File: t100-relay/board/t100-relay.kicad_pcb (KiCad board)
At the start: 2 copper layers, 34.5 x 99.5 mm, 14 parts, among them J1 T100-IN, J2 T100-OUT, J3 Conn_01x02_Female, J4 Conn_01x02_Female, K1 RELAY_2, Q1 BC817, U1 ATSAMD09C13A-SS, X1 SWD

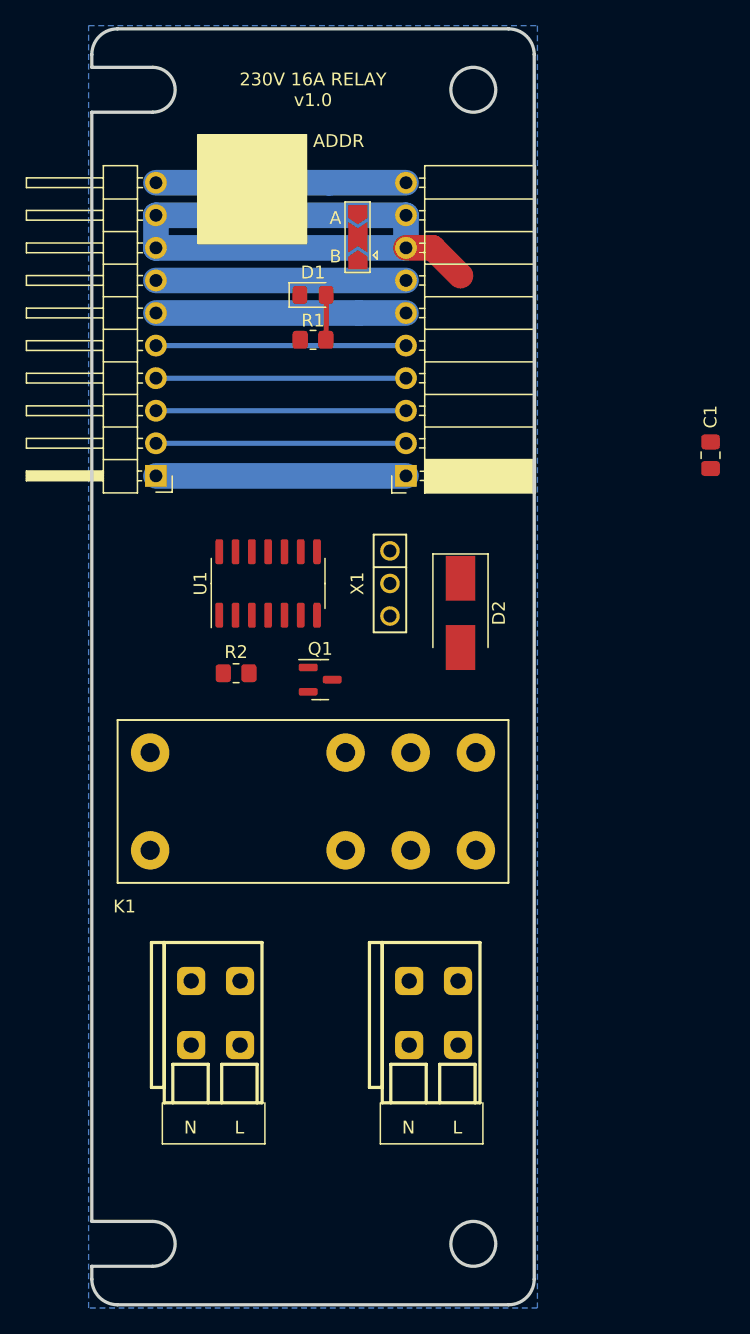
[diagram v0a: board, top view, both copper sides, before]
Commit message: WIP
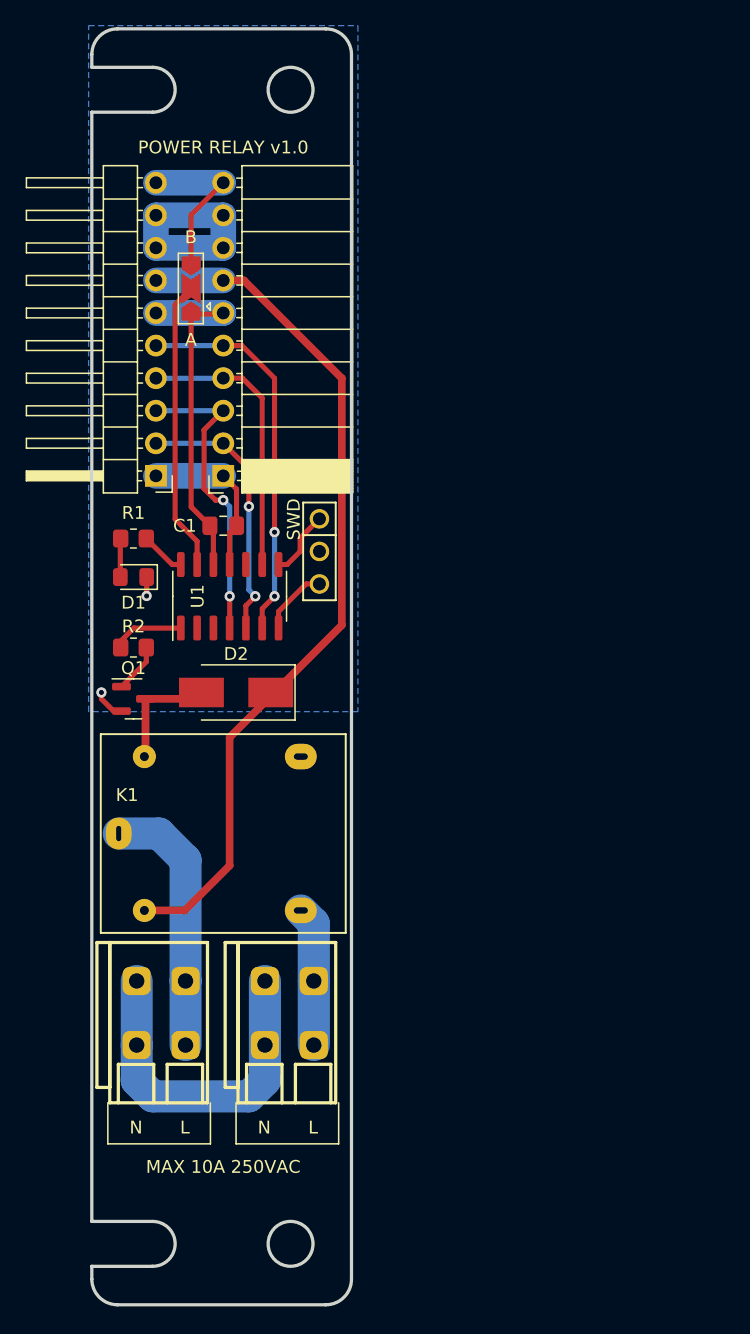
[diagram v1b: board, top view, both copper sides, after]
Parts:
- K1: value RELAY_2 -> RELAY_1; footprint Drake:RT314_Relay -> Drake:SRD_C_Relay
- moved C1 38.4 mm to (93.0, 89.0), turned to 0 degrees
- moved D1 26.1 mm to (86.0, 93.0), turned to 180 degrees
- moved R1 20.9 mm to (86.0, 90.0), turned to 0 degrees
- moved D2 18.6 mm to (94.0, 102.0), turned to 180 degrees
- moved Q1 14.6 mm to (86.0, 102.5)
- moved J2 14.2 mm to (93.0, 85.1)
- moved JP1 13.6 mm to (90.5, 70.5)
- moved J4 11.2 mm to (96.2, 124.5)
- moved R2 8.25 mm to (86.0, 98.5)
- moved X1 6.04 mm to (100.5, 91.0)
- moved J3 4.25 mm to (86.2, 124.5)
- moved U1 3.16 mm to (93.5, 94.5)
- moved K1 2.78 mm to (84.8, 113.0)
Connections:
- K1 pad 2: Net-(D2-Pad2) -> Net-(J4-Pad2)
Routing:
- net +5V: track 19.5 -> 67.6 mm
- net +12V: track 49.2 -> 15.6 mm
- net Net-(J3-Pad1): track 0.00 -> 26.5 mm
- net /ADDR: track 0.00 -> 22.8 mm
- net Net-(J3-Pad2): track 0.00 -> 20.5 mm
- net +3V3: track 19.5 -> 31.7 mm
- net Net-(J4-Pad2): track 0.00 -> 10.9 mm
- net /RST: track 19.5 -> 30.2 mm, vias 0 -> 2
- net GND: track 39.0 -> 29.3 mm, vias 0 -> 2
- net Net-(D2-Pad2): track 0.00 -> 9.11 mm
- net /RELAY: track 0.00 -> 5.61 mm
- net /SWCLK: track 0.00 -> 5.37 mm
- net /SWDIO: track 0.00 -> 5.28 mm
- net /SDA: track 19.5 -> 24.0 mm, vias 0 -> 2
- net Net-(Q1-Pad1): track 0.00 -> 3.85 mm
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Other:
- board size 34.5 x 99.5 mm -> 20.3 x 99.5 mm
- board text added: "MAX 10A 250VAC"
- board text added: "POWER RELAY v1.0"
- board text added: "SWD"
- board text removed: "230V 16A RELAY v1.0"
- board text removed: "ADDR"
